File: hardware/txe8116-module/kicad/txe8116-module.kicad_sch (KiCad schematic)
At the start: 2 parts, among them J1 Screw_Terminal_01x02

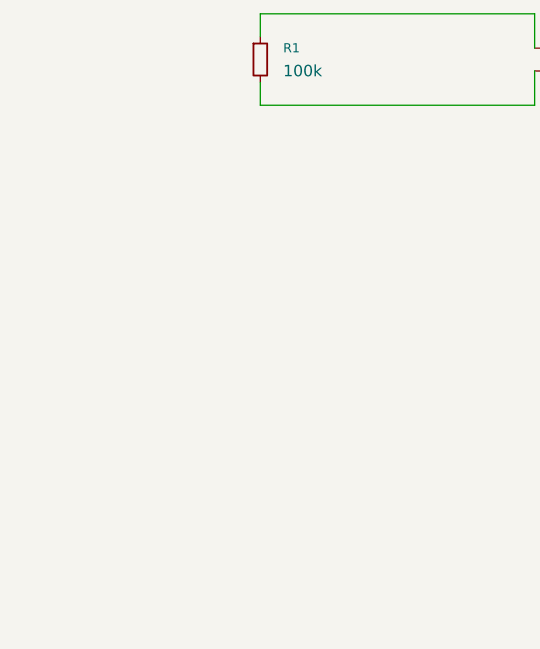
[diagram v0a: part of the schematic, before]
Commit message: Added some components
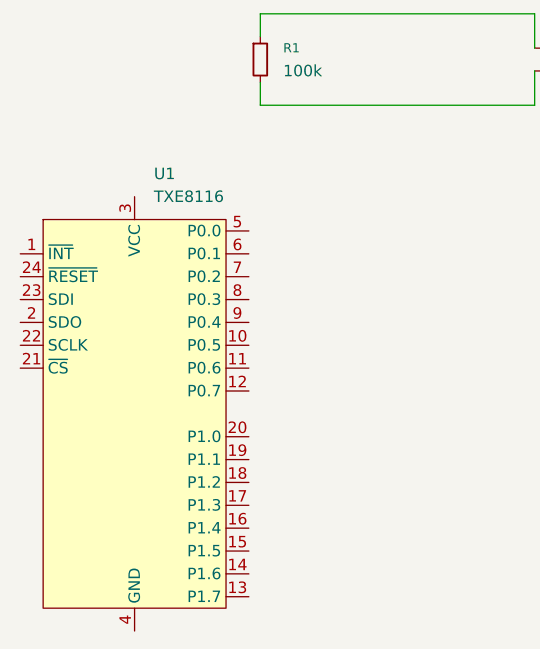
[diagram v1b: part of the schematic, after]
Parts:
- added U1: TXE8116, txe8116:Texas_DGS0024A_TSSOP-24_3x6.1mm_P0.5mm, symbol txe8116:TXE8116
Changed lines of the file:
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@@
+		)
+	)
+	(symbol
+		(lib_id "txe8116:TXE8116")
+		(at 120.65 111.76 0)
+		(unit 1)
+		(exclude_from_sim no)
+		(in_bom yes)
+		(on_board yes)
+		(dnp no)
+		(fields_autoplaced yes)
+		(property "Reference" "U1"
+			(at 122.7933 85.09 0)
+			(effects
+				(font
+					(size 1.27 1.27)
+				)
+				(justify left)
+			)
+		)
+		(property "Value" "TXE8116"
+			(at 122.7933 87.63 0)
+			(effects
+				(font
+					(size 1.27 1.27)
+				)
+				(justify left)
+			)
+		)
+		(property "Footprint" "txe8116:Texas_DGS0024A_TSSOP-24_3x6.1mm_P0.5mm"
+			(at 120.65 111.76 0)
+			(effects
+				(font
+					(size 1.27 1.27)
+				)
+				(hide yes)
+			)
+		)
+		(property "Datasheet" "https://www.ti.com/lit/ds/symlink/txe8116.pdf"
+			(at 120.65 111.76 0)
+			(effects
+				(font
+					(size 1.27 1.27)
+				)
+				(hide yes)
+			)
+		)
+		(property "Description" "16-Bit SPI Bus I/O Expander with Interrupt Output, Reset Input"
+			(at 120.65 111.76 0)
+			(effects
+				(font
+					(size 1.27 1.27)
+				)
+				(hide yes)
+			)
+		)
+		(pin "4"
+		)
+		(pin "6"
+		)
+		(pin "1"
+		)
+		(pin "2"
+		)
+		(pin "24"
+		)
+		(pin "22"
+		)
+		(pin "21"
+		)
+		(pin "3"
+		)
+		(pin "23"
+		)
+		(pin "5"
+		)
+		(pin "19"
+		)
+		(pin "16"
+		)
+		(pin "18"
+		)
+		(pin "15"
+		)
+		(pin "14"
+		)
+		(pin "10"
+		)
+		(pin "12"
+		)
+		(pin "17"
+		)
+		(pin "7"
+		)
+		(pin "13"
+		)
+		(pin "8"
+		)
+		(pin "20"
+		)
+		(pin "9"
+		)
+		(pin "11"
+		)
+		(instances
+			(project ""
+				(path "/07123eb2-095c-4276-b37d-21a84783f032"
+					(reference "U1")
+					(unit 1)
+				)
+			)
 		)
 	)

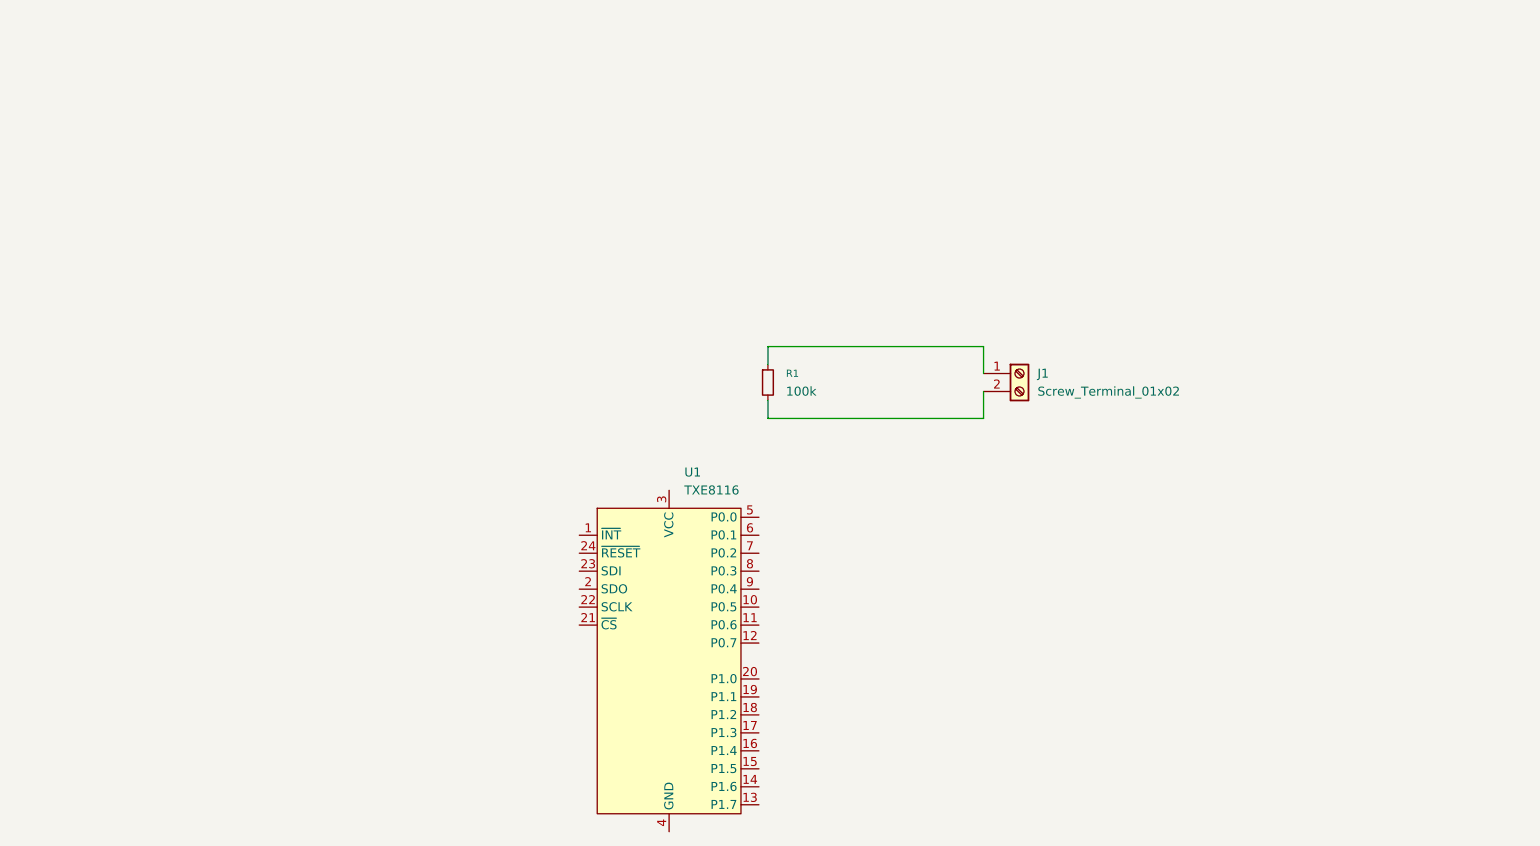
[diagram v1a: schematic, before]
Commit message: Refactor code structure for improved readability and maintainability
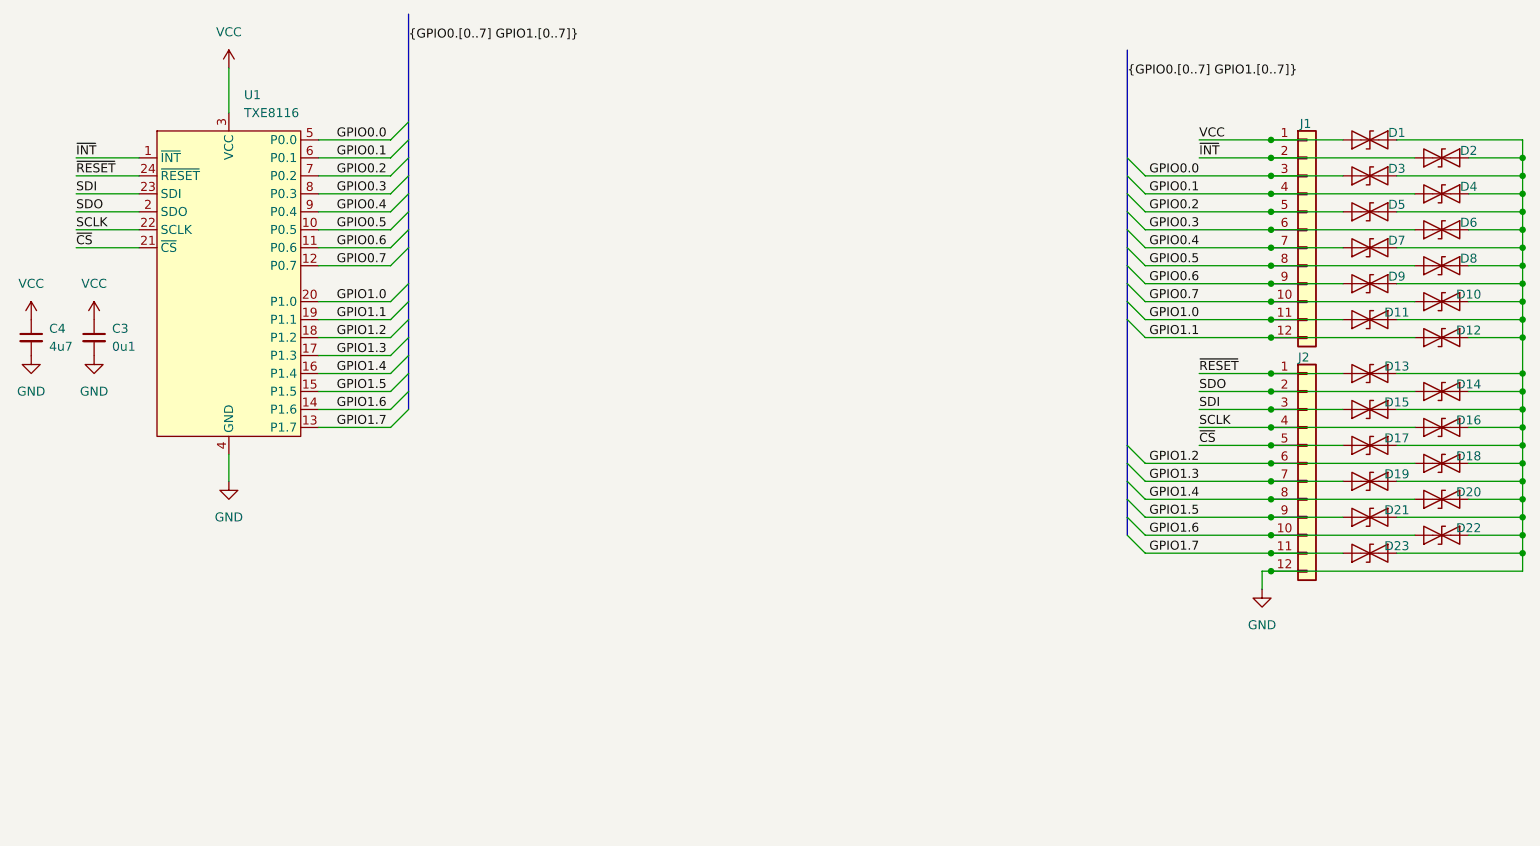
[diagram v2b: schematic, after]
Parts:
- removed J1: Screw_Terminal_01x02, TerminalBlock_WAGO:TerminalBlock_WAGO_2601-1102_1x02_P3.50mm_Horizontal, symbol Connector:Screw_Terminal_01x02
- removed R1: 100k, Resistor_SMD:R_0805_2012Metric, symbol Device:R_Small
- added C3: 0u1, Capacitor_SMD:C_0603_1608Metric, symbol Device:C_Small
- added C4: 4u7, Capacitor_SMD:C_0603_1608Metric, symbol Device:C_Small
- added D1, D10, D11, D12, D13, D14, D15, D16, D17, D18, D19, D2, D20, D21, D22, D23, D3, D4, D5, D6, D7, D8, D9: ESD9B5.0ST5G, Diode_SMD:D_SOD-923, symbol Diode:ESD9B5.0ST5G
- added J1: Conn_01x12, misc:1x12_P2.54mm_Castellated_Mirrored, symbol Connector_Generic:Conn_01x12
- added J2: Conn_01x12, misc:1x12_P2.54mm_Castellated, symbol Connector_Generic:Conn_01x12
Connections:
- net ~{INT}: now reaches U1.1 (~{INT})
- net ~{INT}: now also D2.1 (A1), J1.2 (Pin_2)
- net GPIO0.5: now reaches U1.10 (P0.5)
- net GPIO0.5: now also D8.1 (A1), J1.8 (Pin_8)
- net GPIO0.6: now reaches U1.11 (P0.6)
- net GPIO0.6: now also D9.1 (A1), J1.9 (Pin_9)
- net GPIO0.7: now reaches U1.12 (P0.7)
- net GPIO0.7: now also D10.1 (A1), J1.10 (Pin_10)
- net GPIO1.7: now reaches U1.13 (P1.7)
- net GPIO1.7: now also D23.1 (A1), J2.11 (Pin_11)
- net GPIO1.6: now reaches U1.14 (P1.6)
- net GPIO1.6: now also D22.1 (A1), J2.10 (Pin_10)
- net GPIO1.5: now reaches U1.15 (P1.5)
- net GPIO1.5: now also D21.1 (A1), J2.9 (Pin_9)
- net GPIO1.4: now reaches U1.16 (P1.4)
- net GPIO1.4: now also D20.1 (A1), J2.8 (Pin_8)
- net GPIO1.3: now reaches U1.17 (P1.3)
- net GPIO1.3: now also D19.1 (A1), J2.7 (Pin_7)
- net GPIO1.2: now reaches U1.18 (P1.2)
- net GPIO1.2: now also D18.1 (A1), J2.6 (Pin_6)
- net GPIO1.1: now reaches U1.19 (P1.1)
- net GPIO1.1: now also D12.1 (A1), J1.12 (Pin_12)
- net SDO: now reaches U1.2 (SDO)
- net SDO: now also D14.1 (A1), J2.2 (Pin_2)
- net GPIO1.0: now reaches U1.20 (P1.0)
- net GPIO1.0: now also D11.1 (A1), J1.11 (Pin_11)
- net ~{CS}: now reaches U1.21 (~{CS})
- net ~{CS}: now also D17.1 (A1), J2.5 (Pin_5)
- net SCLK: now reaches U1.22 (SCLK)
- net SCLK: now also D16.1 (A1), J2.4 (Pin_4)
- net SDI: now reaches U1.23 (SDI)
- net SDI: now also D15.1 (A1), J2.3 (Pin_3)
- net ~{RESET}: now reaches U1.24 (~{RESET})
- net ~{RESET}: now also D13.1 (A1), J2.1 (Pin_1)
- net VCC: now reaches U1.3 (VCC)
- net VCC: now also C3.1, C4.1, D1.1 (A1), J1.1 (Pin_1)
- net GND: now reaches U1.4 (GND)
- net GND: now also C3.2, C4.2, D1.2 (A2), D10.2 (A2), D11.2 (A2), D12.2 (A2), D13.2 (A2), D14.2 (A2), D15.2 (A2), D16.2 (A2), D17.2 (A2), D18.2 (A2), D19.2 (A2), D2.2 (A2), D20.2 (A2), D21.2 (A2), D22.2 (A2), D23.2 (A2), D3.2 (A2), D4.2 (A2), D5.2 (A2), D6.2 (A2), D7.2 (A2), D8.2 (A2), D9.2 (A2), J2.12 (Pin_12)
- net GPIO0.0: now reaches U1.5 (P0.0)
- net GPIO0.0: now also D3.1 (A1), J1.3 (Pin_3)
- net GPIO0.1: now reaches U1.6 (P0.1)
- net GPIO0.1: now also D4.1 (A1), J1.4 (Pin_4)
- net GPIO0.2: now reaches U1.7 (P0.2)
- net GPIO0.2: now also D5.1 (A1), J1.5 (Pin_5)
- net GPIO0.3: now reaches U1.8 (P0.3)
- net GPIO0.3: now also D6.1 (A1), J1.6 (Pin_6)
- net GPIO0.4: now reaches U1.9 (P0.4)
- net GPIO0.4: now also D7.1 (A1), J1.7 (Pin_7)
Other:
- moved on the sheet: U1
